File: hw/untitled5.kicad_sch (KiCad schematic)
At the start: 1 part, among them U6 TS3USB3031

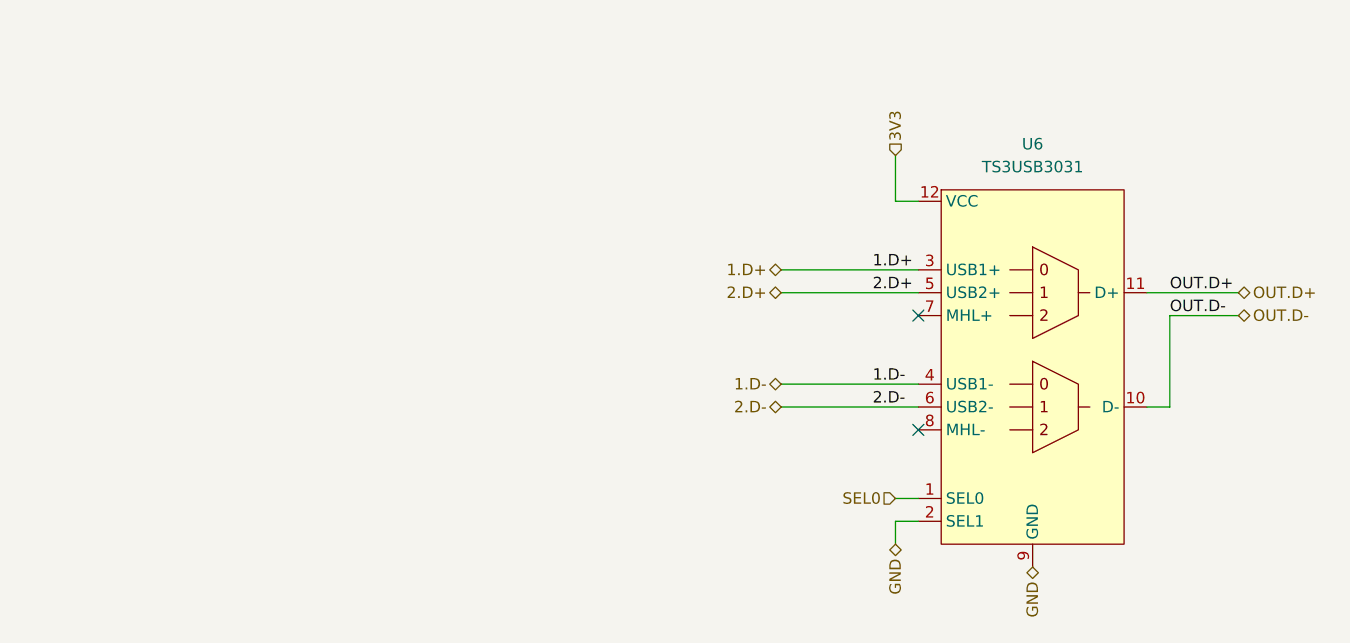
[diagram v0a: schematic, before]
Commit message: add routing
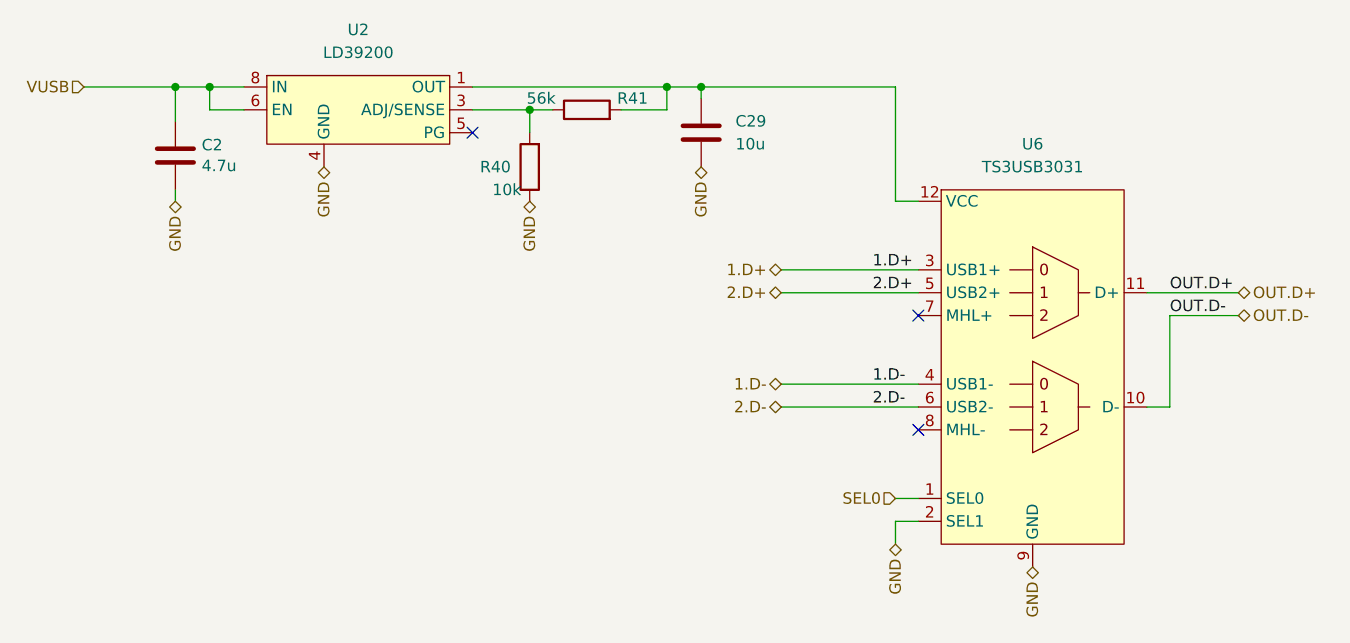
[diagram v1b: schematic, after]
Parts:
- added C2: 4.7u, Capacitor_SMD:C_0603_1608Metric, symbol Device:C
- added C29: 10u, Capacitor_SMD:C_0603_1608Metric, symbol Device:C
- added R40: 10k, Resistor_SMD:R_0402_1005Metric, symbol Device:R
- added R41: 56k, Resistor_SMD:R_0402_1005Metric, symbol Device:R
- added U2: LD39200, Package_DFN_QFN:DFN-8-1EP_4x4mm_P0.8mm_EP2.3x3.24mm, symbol Robotarna_KiCad_Library:LD39200
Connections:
- net GND: now also C2.2, C29.2, R40.1, U2.4 (GND), U2.9 (GND)
- net 3V3: no longer names the net of U6.12 (VCC)
- net 3V3: now also C29.1, R41.2, U2.1 (OUT), U2.2 (OUT)
- new net: R40.2, R41.1, U2.3 (ADJ/SENSE)
- new net IN: C2.1, U2.6 (EN), U2.7 (IN), U2.8 (IN)
- no-connect marks 2 -> 3
